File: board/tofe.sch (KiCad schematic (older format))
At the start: 16 parts

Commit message: Lots of small fixes to the schematic.
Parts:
- added DDG4: LED, LEDs:LED_0805, symbol LED
- added RDG4: 68R, Resistors_SMD:R_0805_HandSoldering, symbol R
- PDG0: symbol CONN_02X05 -> CONN_02X06
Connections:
- net +3V3: now also PDG0.11 (P11), PDG0.12 (P12), DDG4.2 (A); no longer PDG0.2 (P2)
- net GND: now also PDG0.9 (P9)
- net IDDAT: now also PDG0.1 (P1)
- net at RDG1.2: now also PDG0.2 (P2); no longer PDG0.4 (P4)
- net at RDG2.2: now also PDG0.4 (P4); no longer PDG0.6 (P6)
- net at RDG3.2: now also PDG0.6 (P6); no longer PDG0.8 (P8)
- net VGAIN_I2C_EN: no longer names the net of PDG0.3 (P3), TOFE0.B9 (DIFF_IO_XP)
- net VGAOUT_I2C_EN: no longer names the net of PDG0.5 (P5), TOFE0.B11 (DIFF_IO_XN)
- new net: PDG0.8 (P8), RDG4.2
- new net: DDG4.1 (K), RDG4.1
- no-connect marks 5 -> 3
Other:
- moved on the sheet: DDG1, DDG2, DDG3, RDG1, RDG2, RDG3

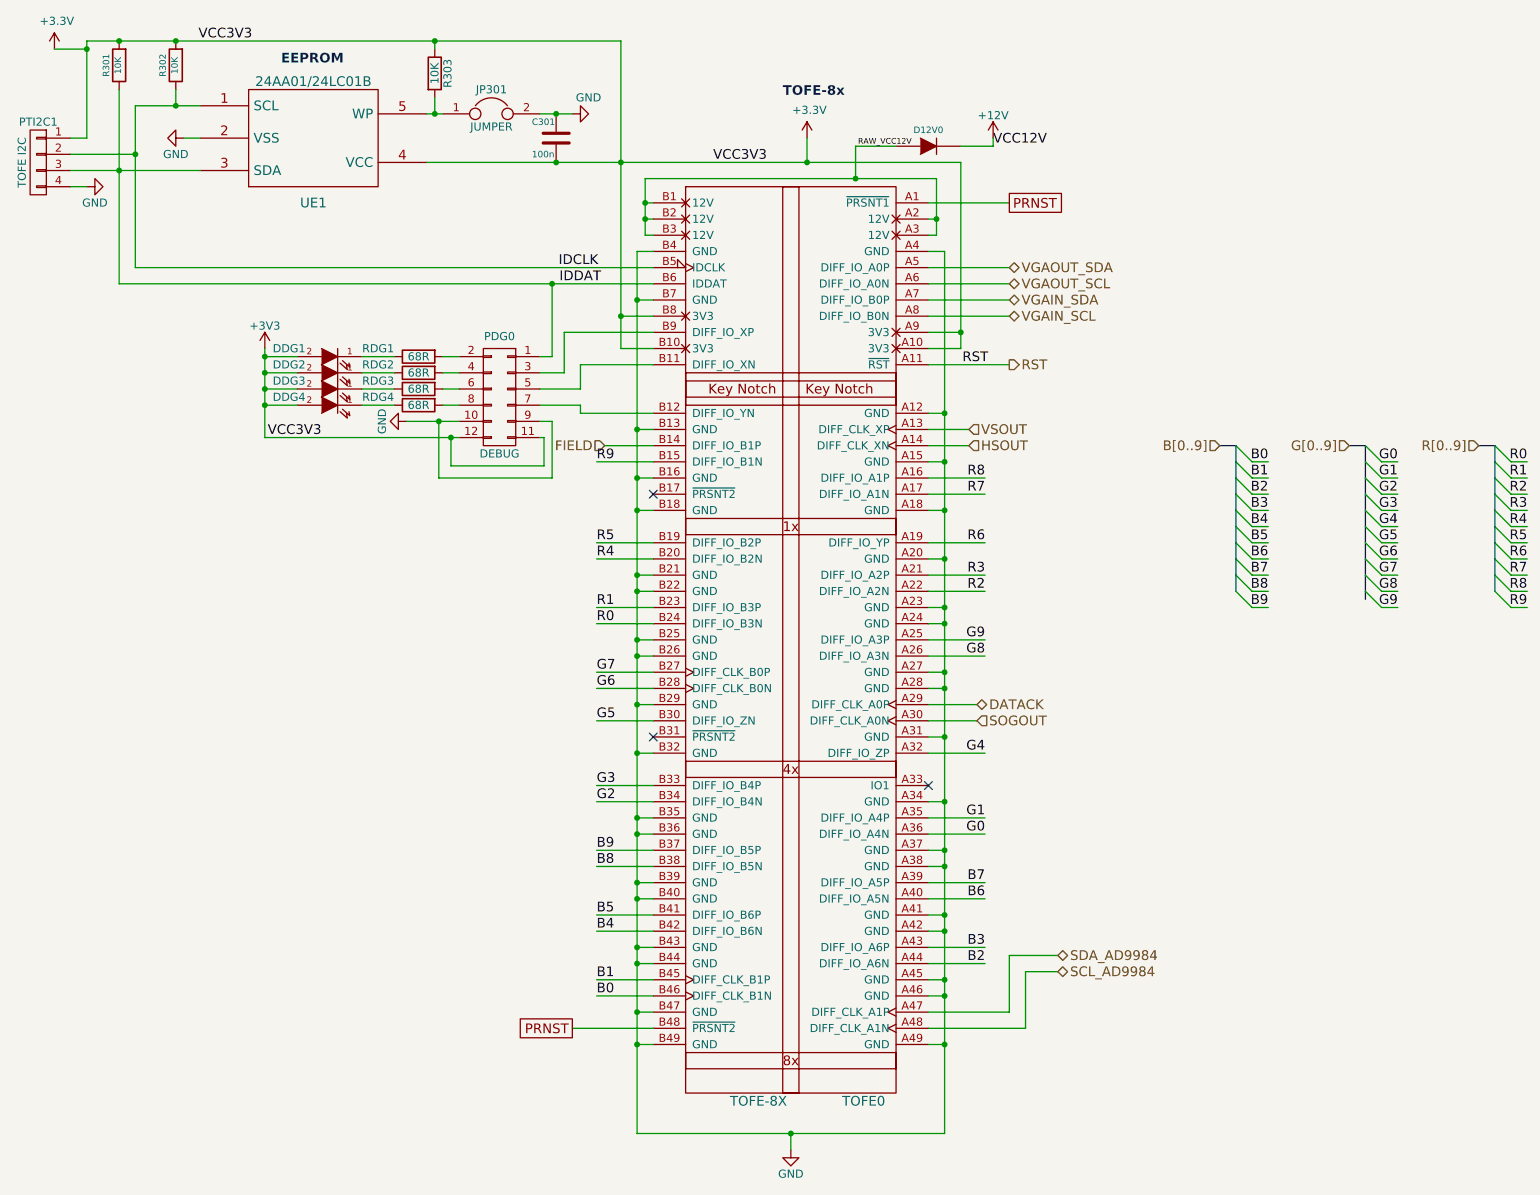
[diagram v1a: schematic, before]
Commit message: Lots of small fixes.
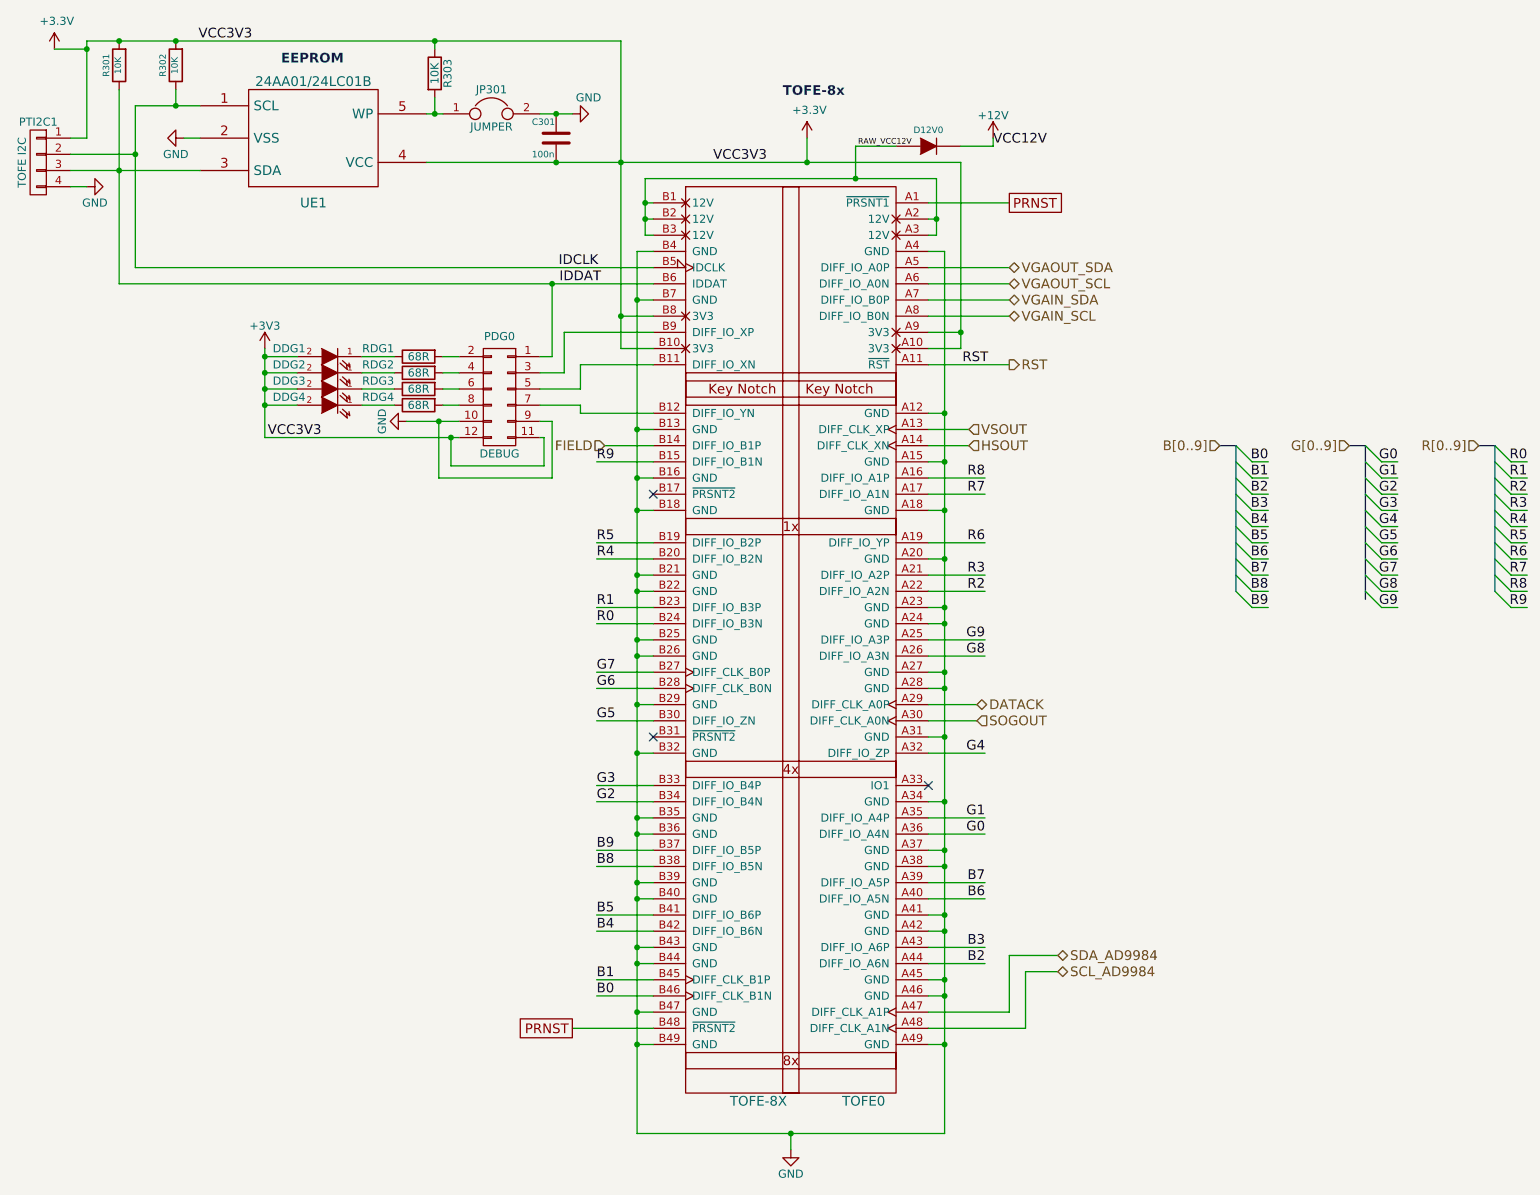
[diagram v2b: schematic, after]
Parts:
- PDG0: footprint Pin_Headers:Pin_Header_Straight_2x05 -> Pin_Headers:Pin_Header_Straight_2x06
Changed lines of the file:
@@
 F 0 "PDG0" H 3650 3225 50  0000 C CNN
 F 1 "DEBUG" H 3650 2500 50  0000 C CNN
-F 2 "Pin_Headers:Pin_Header_Straight_2x05" H 3650 1650 50  0001 C CNN
+F 2 "Pin_Headers:Pin_Header_Straight_2x06" H 3650 1650 50  0001 C CNN
 F 3 "" H 3650 1650 50  0000 C CNN
 	1    3650 2850
@@
 	4600 1950 4500 1950
 Wire Wire Line
-	4500 1950 4500 2250
-Wire Wire Line
-	4500 2250 4500 3050
-Wire Wire Line
-	4500 3050 4500 3350
-Wire Wire Line
-	4500 3350 4500 3550
-Wire Wire Line
-	4500 3550 4500 3950
-Wire Wire Line
-	4500 3950 4500 4050
-Wire Wire Line
-	4500 4050 4500 4350
-Wire Wire Line
-	4500 4350 4500 4450
-Wire Wire Line
-	4500 4450 4500 4750
-Wire Wire Line
-	4500 4750 4500 5050
-Wire Wire Line
-	4500 5050 4500 5450
-Wire Wire Line
-	4500 5450 4500 5550
-Wire Wire Line
-	4500 5550 4500 5850
-Wire Wire Line
-	4500 5850 4500 5950
-Wire Wire Line
-	4500 5950 4500 6250
-Wire Wire Line
-	4500 6250 4500 6350
-Wire Wire Line
-	4500 6350 4500 6650
-Wire Wire Line
-	4500 6650 4500 6850
-Wire Wire Line
-	4500 6850 4500 7400
+	4500 1950 4500 7400
 Wire Wire Line
 	4500 2250 4600 2250
@@
 Connection ~ 6400 6550
 Wire Wire Line
-	4500 7400 5450 7400
-Wire Wire Line
-	5450 7400 6400 7400
+	4500 7400 6400 7400
 Connection ~ 4500 6850
 Connection ~ 6400 6850
@@
 	4400 2550 4600 2550
 Wire Wire Line
-	4400 650  4400 1400
-Wire Wire Line
-	4400 1400 4400 2350
-Wire Wire Line
-	4400 2350 4400 2550
+	4400 650  4400 2550
 Wire Wire Line
 	4400 2350 4600 2350
@@
 	6300 2450 6500 2450
 Wire Wire Line
-	6500 1400 6500 2450
-Wire Wire Line
-	6500 2450 6500 2550
+	6500 1400 6500 2550
 Wire Wire Line
 	6500 2550 6300 2550
 Wire Wire Line
-	3200 1400 4000 1400
-Wire Wire Line
-	4000 1400 4400 1400
-Wire Wire Line
-	4400 1400 5550 1400
-Wire Wire Line
-	5550 1400 6500 1400
+	3200 1400 6500 1400
 Connection ~ 6500 2450
 Connection ~ 4400 2350
@@
 	4550 1850 4600 1850
 Wire Wire Line
-	4550 1500 4550 1650
-Wire Wire Line
-	4550 1650 4550 1750
-Wire Wire Line
-	4550 1750 4550 1850
+	4550 1500 4550 1850
 Wire Wire Line
 	4550 1750 4600 1750
@@
 	6350 1850 6300 1850
 Wire Wire Line
-	6350 1500 6350 1750
-Wire Wire Line
-	6350 1750 6350 1850
+	6350 1500 6350 1850
 Wire Wire Line
 	6350 1750 6300 1750
 Wire Wire Line
-	4550 1500 5850 1500
-Wire Wire Line
-	5850 1500 6350 1500
+	4550 1500 6350 1500
 Connection ~ 6350 1750
 Connection ~ 4550 1650
@@
 Connection ~ 4000 1400
 Wire Wire Line
-	6400 7400 6400 6850
-Wire Wire Line
-	6400 6850 6400 6550
-Wire Wire Line
-	6400 6550 6400 6450
-Wire Wire Line
-	6400 6450 6400 6150
-Wire Wire Line
-	6400 6150 6400 6050
-Wire Wire Line
-	6400 6050 6400 5750
-Wire Wire Line
-	6400 5750 6400 5650
-Wire Wire Line
-	6400 5650 6400 5350
-Wire Wire Line
-	6400 5350 6400 4950
-Wire Wire Line
-	6400 4950 6400 4650
-Wire Wire Line
-	6400 4650 6400 4550
-Wire Wire Line
-	6400 4550 6400 4250
-Wire Wire Line
-	6400 4250 6400 4150
-Wire Wire Line
-	6400 4150 6400 3850
-Wire Wire Line
-	6400 3850 6400 3550
-Wire Wire Line
-	6400 3550 6400 3250
-Wire Wire Line
-	6400 3250 6400 2950
-Wire Wire Line
-	6400 2950 6400 1950
+	6400 7400 6400 1950
 Wire Wire Line
 	1400 2050 4600 2050
 Wire Wire Line
-	1300 2150 3975 2150
-Wire Wire Line
-	3975 2150 4600 2150
-Wire Wire Line
-	3900 1100 4000 1100
-Wire Wire Line
-	4000 1100 4100 1100
+	1300 2150 4600 2150
+Wire Wire Line
+	3900 1100 4100 1100
 Wire Wire Line
 	1700 1250 1800 1250
@@
 	1650 950  1650 1050
 Wire Wire Line
-	1400 1050 1650 1050
-Wire Wire Line
-	1650 1050 1800 1050
-Wire Wire Line
-	1000 1450 1300 1450
-Wire Wire Line
-	1300 1450 1800 1450
+	1400 1050 1800 1050
+Wire Wire Line
+	1000 1450 1800 1450
 Connection ~ 4000 1100
 Wire Wire Line
-	1400 1050 1400 1350
-Wire Wire Line
-	1400 1350 1400 2050
+	1400 1050 1400 2050
 Connection ~ 1650 1050
 Wire Wire Line
-	1100 650  1300 650
-Wire Wire Line
-	1300 650  1650 650
-Wire Wire Line
-	1650 650  3250 650
-Wire Wire Line
-	3250 650  4400 650
+	1100 650  4400 650
 Connection ~ 4400 1400
 Connection ~ 1650 650
@@
 	9700 3150 9800 3150
 Wire Bus Line
-	9800 3150 9800 3250
-Wire Bus Line
-	9800 3250 9800 3350
-Wire Bus Line
-	9800 3350 9800 3450
-Wire Bus Line
-	9800 3450 9800 3550
-Wire Bus Line
-	9800 3550 9800 3650
-Wire Bus Line
-	9800 3650 9800 3750
-Wire Bus Line
-	9800 3750 9800 3850
-Wire Bus Line
-	9800 3850 9800 3950
-Wire Bus Line
-	9800 3950 9800 4050
+	9800 3150 9800 4050
 Wire Bus Line
 	8900 3150 9000 3150
 Wire Bus Line
-	9000 3150 9000 3250
-Wire Bus Line
-	9000 3250 9000 3350
-Wire Bus Line
-	9000 3350 9000 3450
-Wire Bus Line
-	9000 3450 9000 3550
-Wire Bus Line
-	9000 3550 9000 3650
-Wire Bus Line
-	9000 3650 9000 3750
-Wire Bus Line
-	9000 3750 9000 3850
-Wire Bus Line
-	9000 3850 9000 3950
-Wire Bus Line
-	9000 3950 9000 4050
-Wire Bus Line
-	9000 4050 9000 4100
+	9000 3150 9000 4100
 Wire Wire Line
 	6300 5950 6650 5950
@@
 	9200 3550 9100 3550
 Wire Bus Line
-	8200 3150 8200 3250
-Wire Bus Line
-	8200 3250 8200 3350
-Wire Bus Line
-	8200 3350 8200 3450
-Wire Bus Line
-	8200 3450 8200 3550
-Wire Bus Line
-	8200 3550 8200 3650
-Wire Bus Line
-	8200 3650 8200 3750
-Wire Bus Line
-	8200 3750 8200 3850
-Wire Bus Line
-	8200 3850 8200 3950
-Wire Bus Line
-	8200 3950 8200 4050
+	8200 3150 8200 4050
 Wire Wire Line
 	6300 3950 6650 3950
@@
 	6300 4050 6650 4050
 Wire Wire Line
-	3200 1100 3250 1100
-Wire Wire Line
-	3250 1100 3300 1100
-Wire Wire Line
-	1300 950  1300 1450
-Wire Wire Line
-	1300 1450 1300 2150
+	3200 1100 3300 1100
+Wire Wire Line
+	1300 950  1300 2150
 Connection ~ 1300 1450
 Wire Wire Line
@@
 Connection ~ 2200 2600
 Wire Wire Line
-	1100 650  1100 700
-Wire Wire Line
-	1100 700  1100 1250
+	1100 650  1100 1250
 Wire Wire Line
 	1100 1250 1000 1250
@@
 	2200 2800 2400 2800
 Wire Wire Line
-	2200 2550 2200 2600
-Wire Wire Line
-	2200 2600 2200 2700
-Wire Wire Line
-	2200 2700 2200 2800
-Wire Wire Line
-	2200 2800 2200 2900
-Wire Wire Line
-	2200 2900 2200 3100
-Wire Wire Line
-	3075 3000 3275 3000
-Wire Wire Line
-	3275 3000 3400 3000
+	2200 2550 2200 3100
+Wire Wire Line
+	3075 3000 3400 3000
 Wire Wire Line
 	4150 2650 4600 2650
@@
 	4150 2650 4150 2800
 Wire Wire Line
-	2200 3100 3350 3100
-Wire Wire Line
-	3350 3100 3400 3100
+	2200 3100 3400 3100
 Connection ~ 2200 2800
 Wire Wire Line
